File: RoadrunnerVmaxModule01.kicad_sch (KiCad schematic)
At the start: 3 parts, among them M1 Module-power_12and5V-0.3, M2 Module-mega-mcu144-0.7, M3 Module-input-0.1

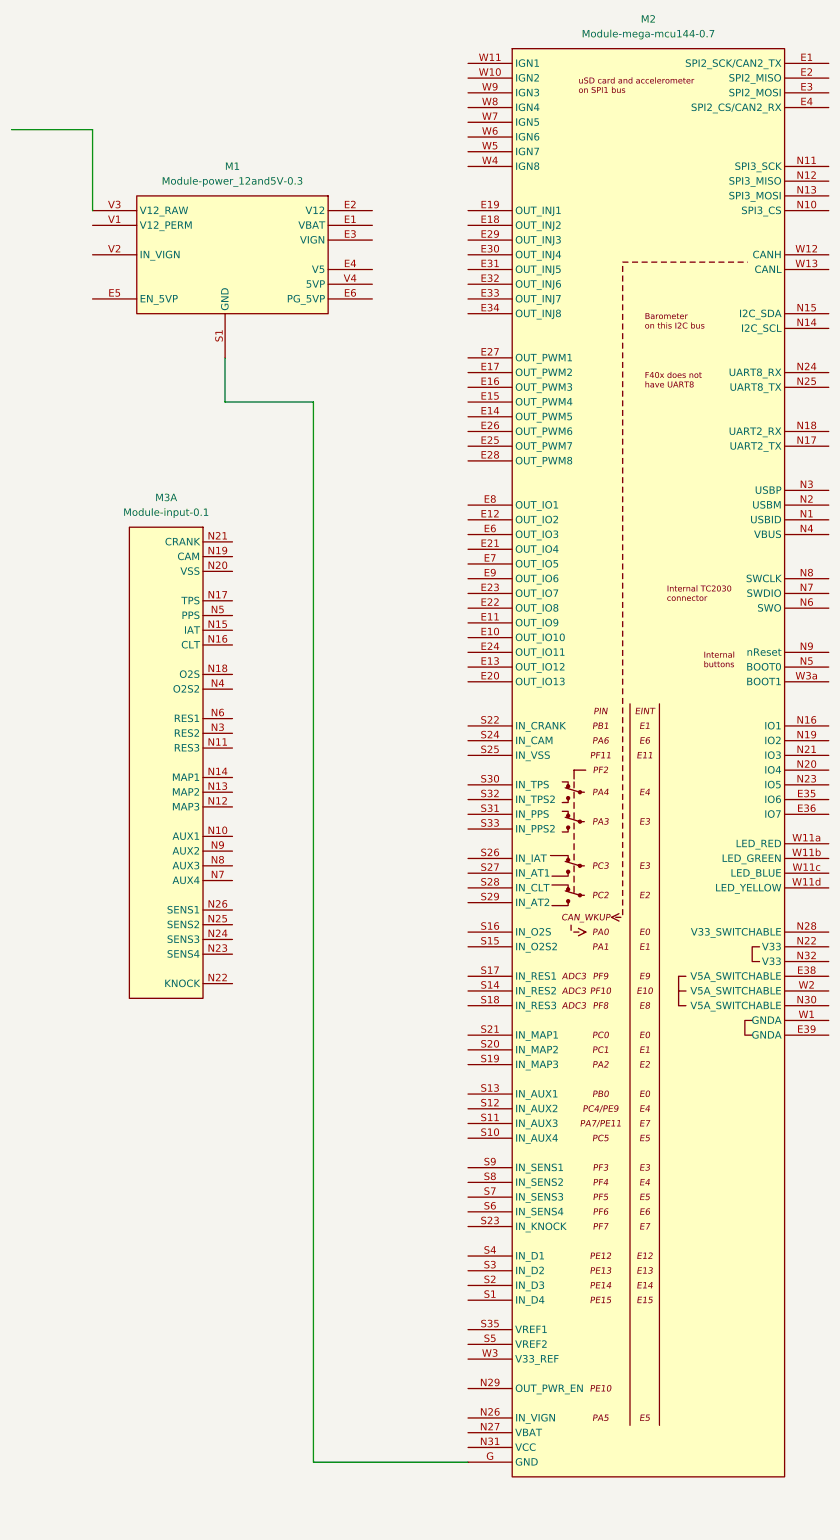
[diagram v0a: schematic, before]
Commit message: 5
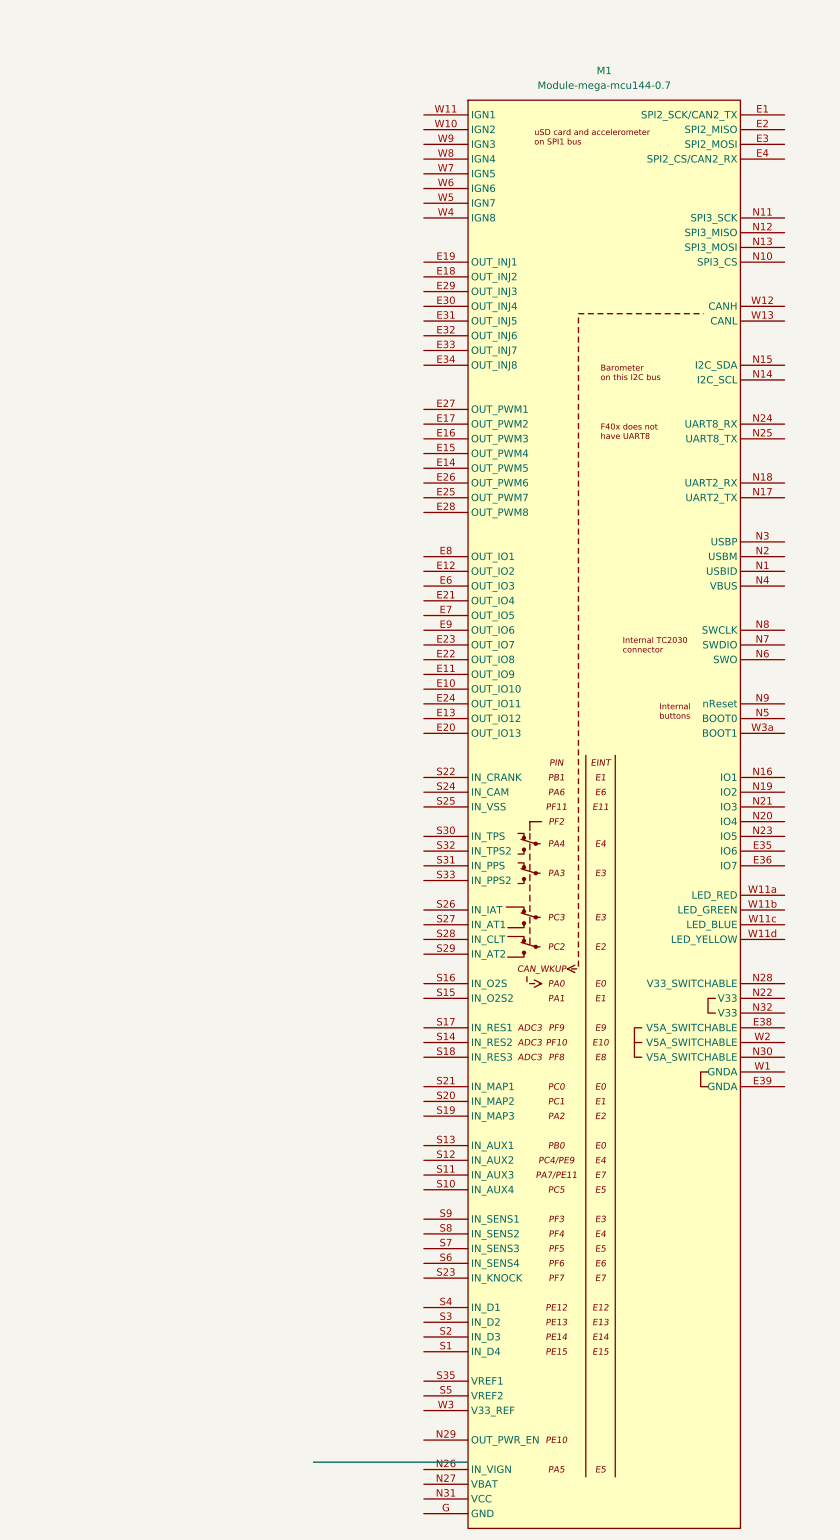
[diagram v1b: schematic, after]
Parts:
- removed M1: Module-power_12and5V-0.3, 0.3:power_12and5V, symbol power_12and5V:Module-power_12and5V-0.3
- removed M2: Module-mega-mcu144-0.7, 0.7:mega-mcu144, symbol mega-mcu144:Module-mega-mcu144-0.7
- removed M3: Module-input-0.1, 0.1:input, symbol input:Module-input-0.1
- added M1: Module-mega-mcu144-0.7, 0.7:mega-mcu144, symbol mega-mcu144:Module-mega-mcu144-0.7
